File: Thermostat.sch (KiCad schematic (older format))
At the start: 21 parts, among them P1 PWR, P2 NTC probe 8K, P3 HEATER, U1 LM358, U2 MOC3063M, U3 TRIAC

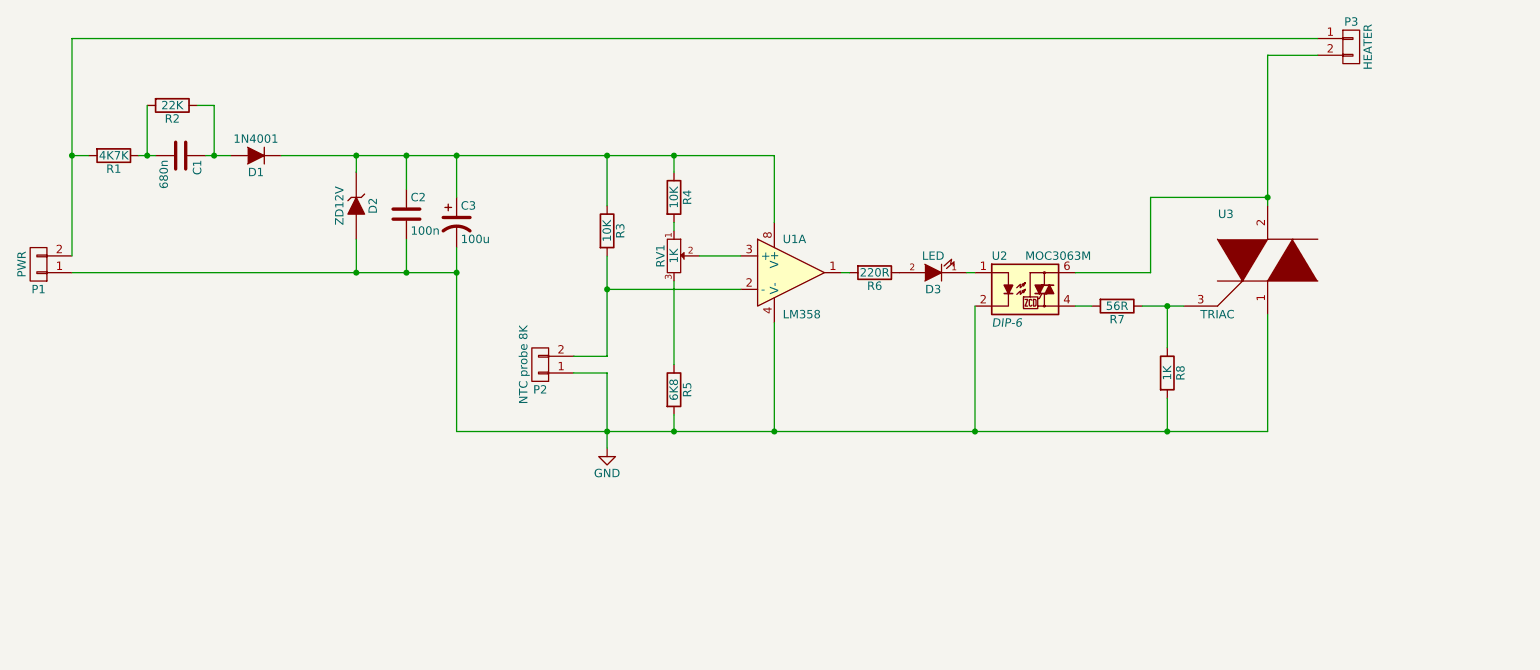
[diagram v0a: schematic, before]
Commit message: Updated schematic
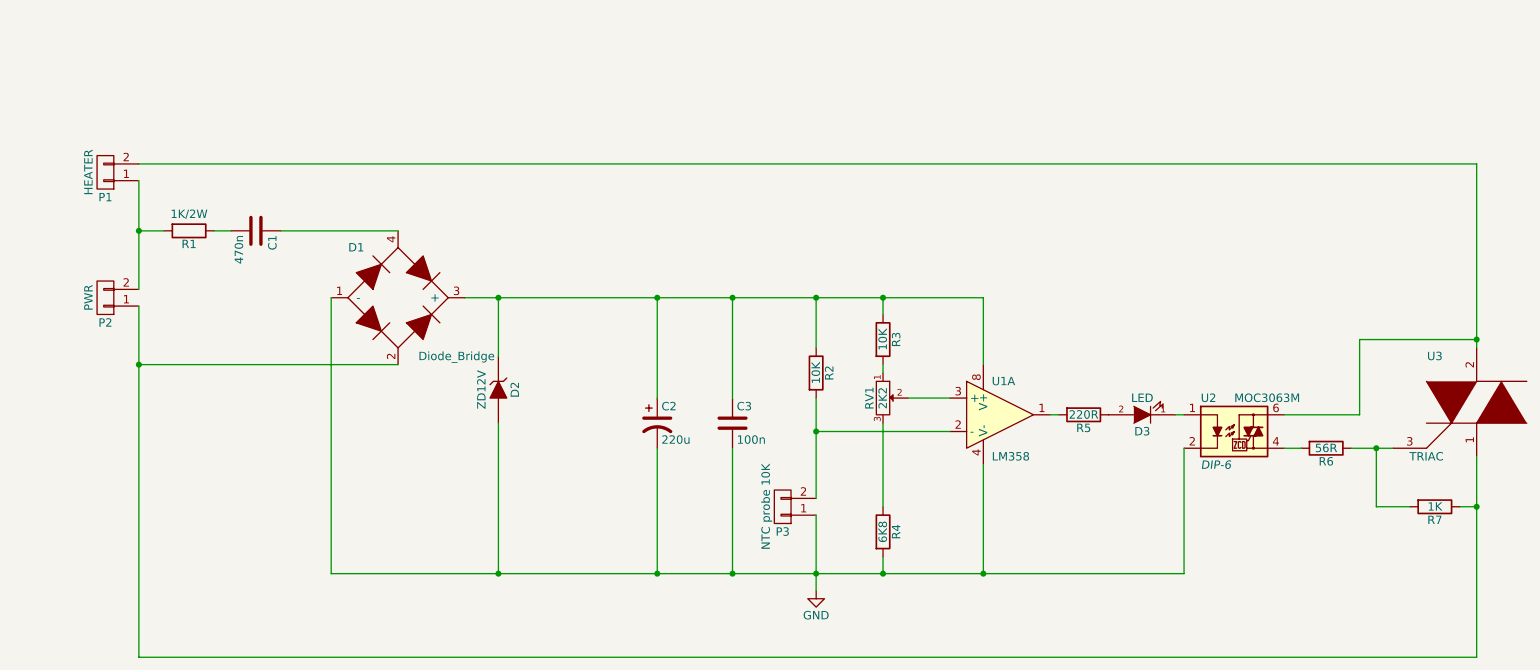
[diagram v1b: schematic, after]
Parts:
- removed D1: 1N4001, symbol D
- removed R2: 22K, symbol R
- added D1: Diode_Bridge, symbol Diode_Bridge
- C1: value 680n -> 470n; footprint (none) -> Capacitors_ThroughHole:C_Rect_L13.5mm_W5.0mm_P10.00mm_FKS3_FKP3_MKS4
- C2: renamed from C3; value 100u -> 220u
- C3: renamed from C2; footprint (none) -> Capacitors_SMD:C_1206_HandSoldering
- P3: renamed from P2; value NTC probe 8K -> NTC probe 10K
- R1: value 4K7K -> 1K/2W
- RV1: value 1K -> 2K2
- renumbered P3 to P1, P1 to P2, R3 to R2, R4 to R3, R5 to R4, R6 to R5, R7 to R6, R8 to R7
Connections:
- net GND: now also D1.1 (-); no longer P2.1 (P1), R7.2, U3.1
- net at C2.1, C3.1, D2.1 (K)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: now also D1.3 (+)
- net at R6.1, U3.3: now also R7.2; no longer R7.1
- net at C1.1: now also D1.4
- new net: D1.2, P2.1 (P1), R7.1, U3.1
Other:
- moved on the sheet: C1, C2, C3, D2, D3, P1, P2, P3, R1, R2, R3, R4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
